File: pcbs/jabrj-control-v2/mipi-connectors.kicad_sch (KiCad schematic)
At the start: 7 parts, among them J901 FH12-22S-0.5SH, J902 FH12-22S-0.5SH

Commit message: 895 Unrouted
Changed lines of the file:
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@@
+		)
+	)
+	(bus
+		(pts
+			(xy 88.9 71.12) (xy 88.9 73.66)
+		)
+		(stroke
+			(width 0)
+			(type default)
 		)
 	)
@@
 	(bus
 		(pts
-			(xy 88.9 71.12) (xy 88.9 73.66)
-		)
-		(stroke
-			(width 0)
-			(type default)
-		)
-	)
-	(bus
-		(pts
 			(xy 88.9 116.84) (xy 88.9 119.38)
 		)
@@
 		)
 	)
+	(bus
+		(pts
+			(xy 88.9 71.12) (xy 91.44 71.12)
+		)
+		(stroke
+			(width 0)
+			(type default)
+		)
+	)
 	(wire
 		(pts
@@
 		(pts
 			(xy 172.72 93.98) (xy 172.72 101.6)
-		)
-		(stroke
-			(width 0)
-			(type default)
-		)
-	)
-	(bus
-		(pts
-			(xy 91.44 71.12) (xy 88.9 71.12)
 		)
 		(stroke
@@
 		)
 	)
+	(netclass_flag ""
+		(length 2.54)
+		(shape round)
+		(at 198.12 71.12 0)
+		(fields_autoplaced yes)
+		(effects
+			(font
+				(size 1.27 1.27)
+			)
+			(justify left bottom)
+		)
+		(property "Net Class" "MIPI"
+			(at 198.8185 68.58 0)
+			(show_name no)
+			(do_not_autoplace no)
+			(effects
+				(font
+					(size 1.27 1.27)
+				)
+				(justify left)
+			)
+		)
+		(property "Component Class" ""
+			(at -78.74 -25.4 0)
+			(show_name no)
+			(do_not_autoplace no)
+			(effects
+				(font
+					(size 1.27 1.27)
+					(italic yes)
+				)
+			)
+		)
+	)
+	(netclass_flag ""
+		(length 2.54)
+		(shape round)
+		(at 88.9 71.12 0)
+		(fields_autoplaced yes)
+		(effects
+			(font
+				(size 1.27 1.27)
+			)
+			(justify left bottom)
+		)
+		(property "Net Class" "MIPI"
+			(at 89.5985 68.58 0)
+			(show_name no)
+			(do_not_autoplace no)
+			(effects
+				(font
+					(size 1.27 1.27)
+				)
+				(justify left)
+			)
+		)
+		(property "Component Class" ""
+			(at -187.96 -25.4 0)
+			(show_name no)
+			(do_not_autoplace no)
+			(effects
+				(font
+					(size 1.27 1.27)
+					(italic yes)
+				)
+			)
+		)
+	)

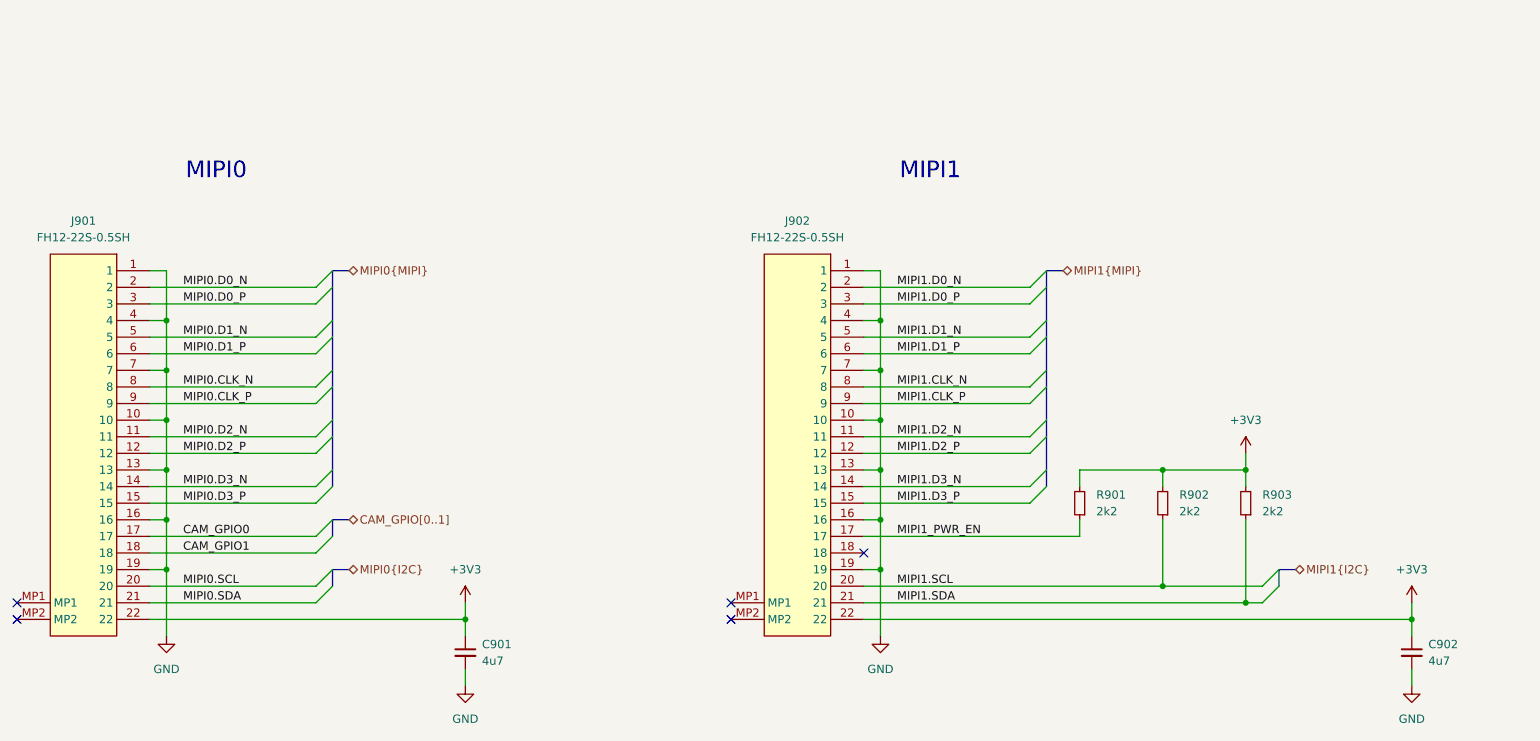
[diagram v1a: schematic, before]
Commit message: 651 Unrouted
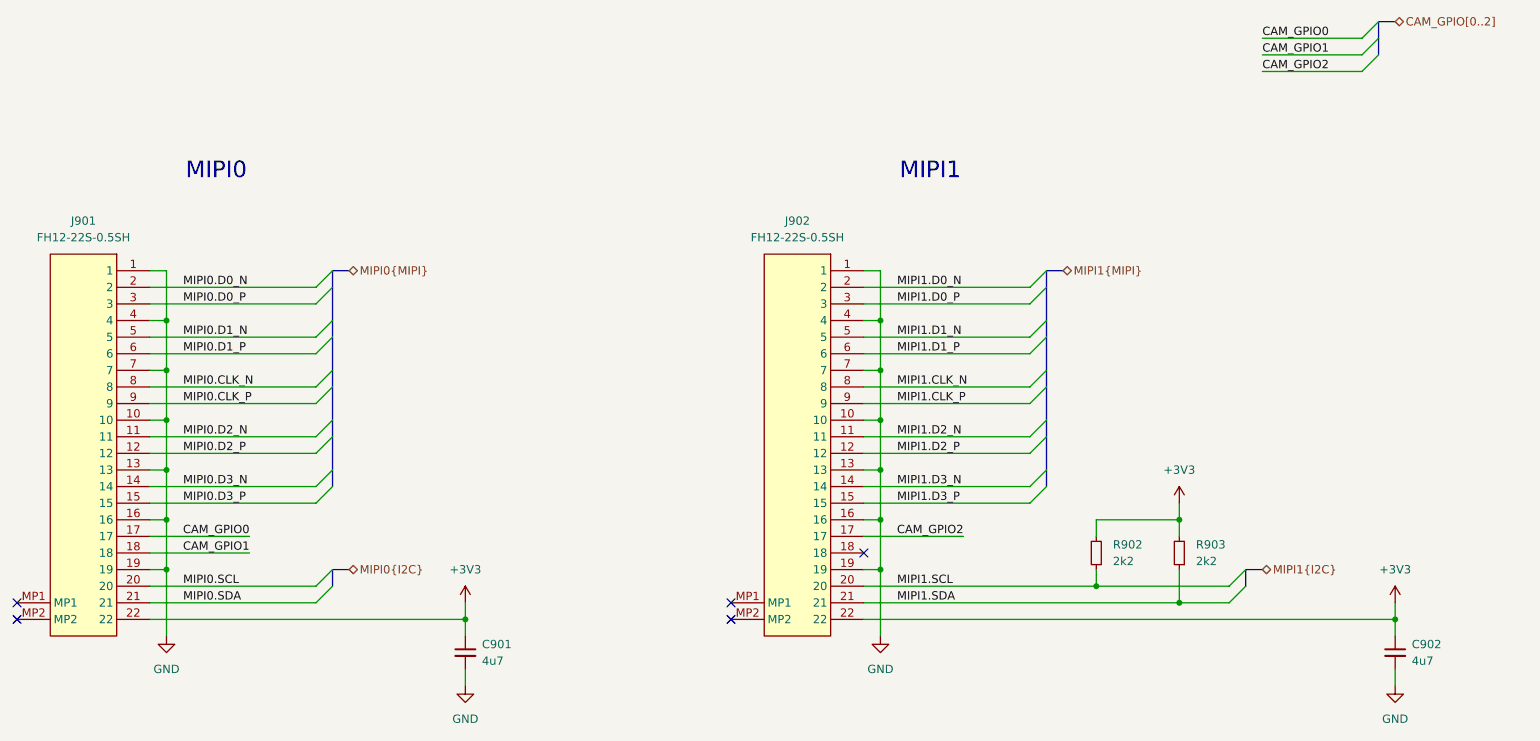
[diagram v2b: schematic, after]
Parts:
- removed R901: 2k2, project_footprints:R_0402, symbol DEV:R_SMALL
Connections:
- net MIPI1_PWR_EN renamed CAM_GPIO2
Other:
- moved on the sheet: C902, R902, R903
